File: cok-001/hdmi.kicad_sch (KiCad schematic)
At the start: 73 parts, among them J2501 HDMI_A, Q2502 DTA144E, Q2504 DTA144E, Q2507 DTC144E

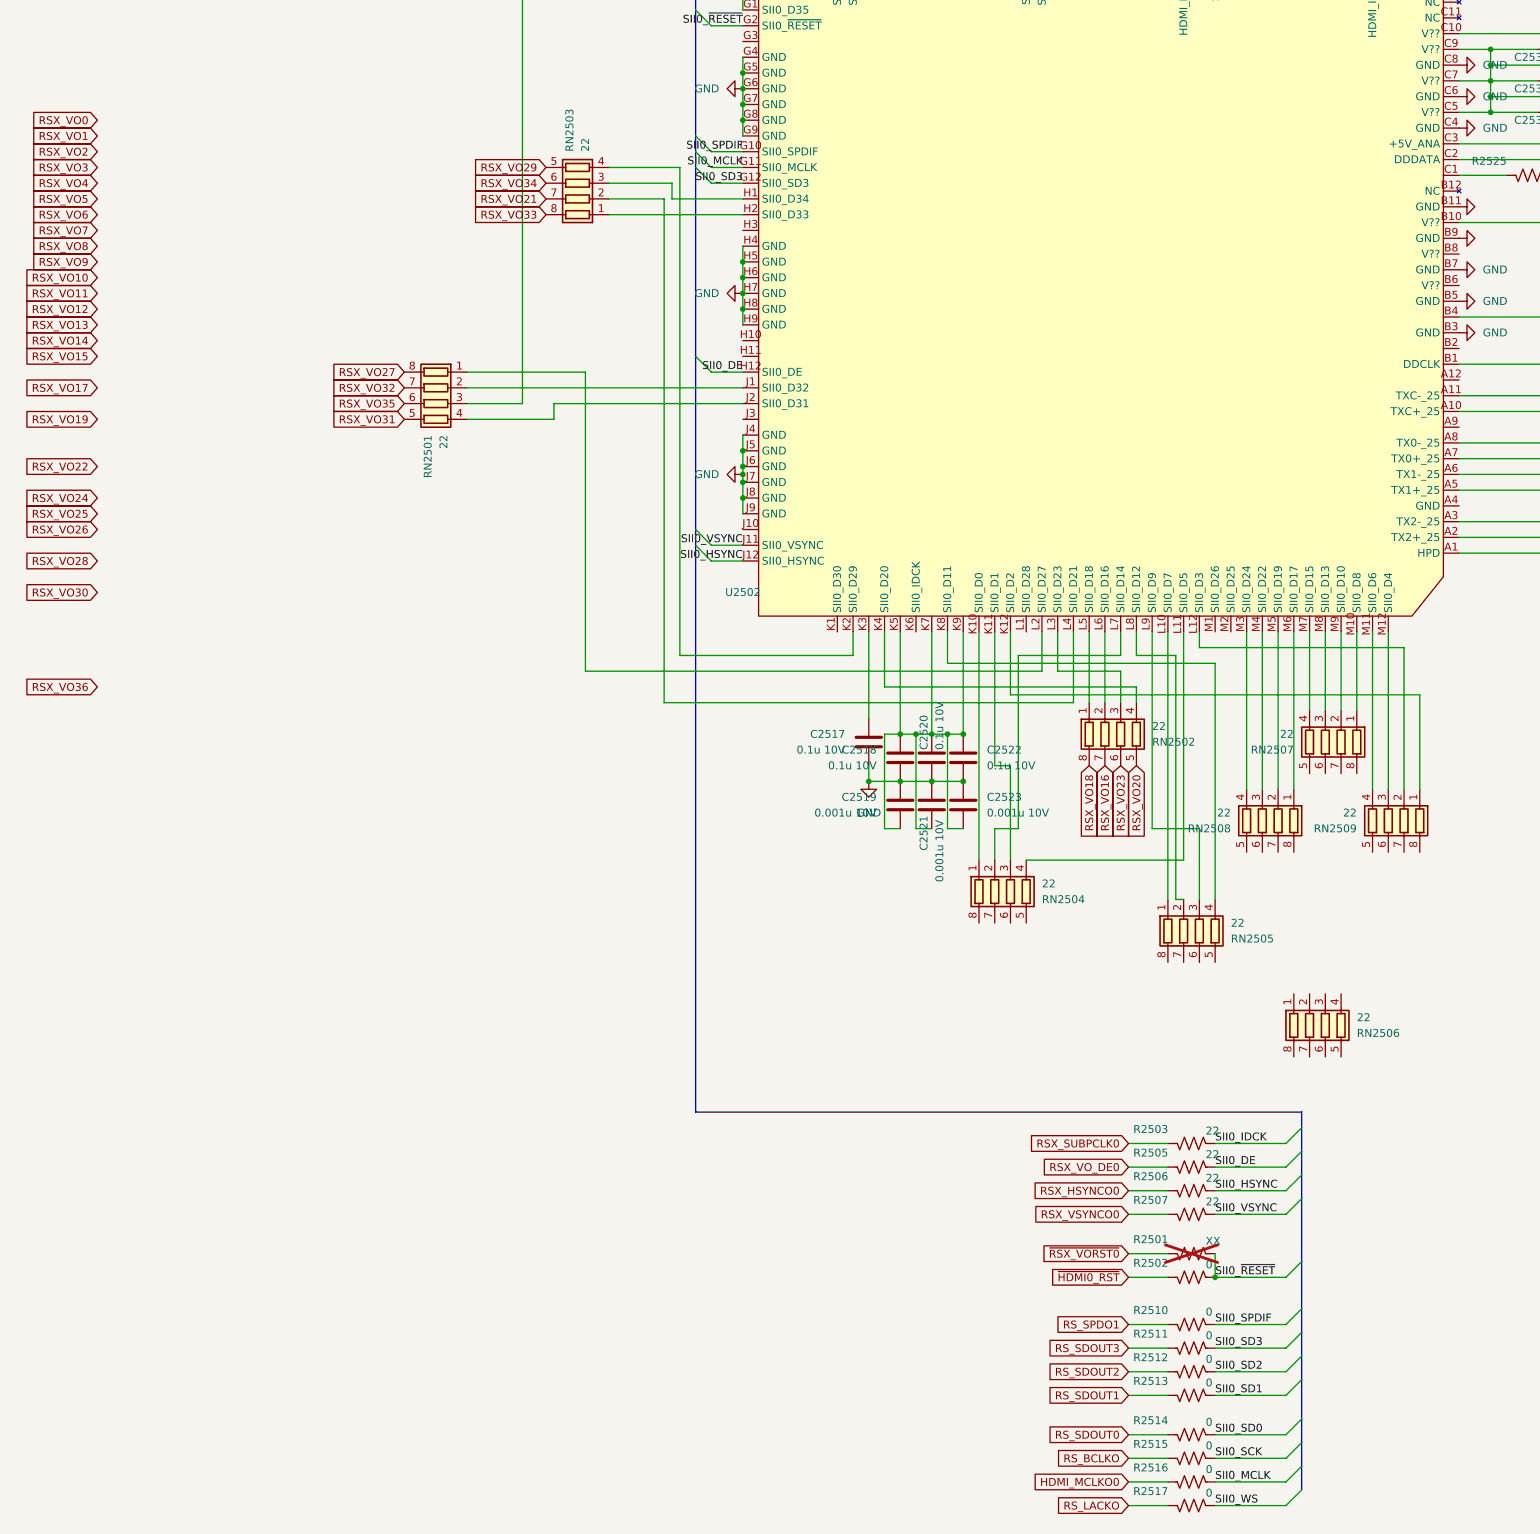
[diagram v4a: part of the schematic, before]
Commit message: hd sb
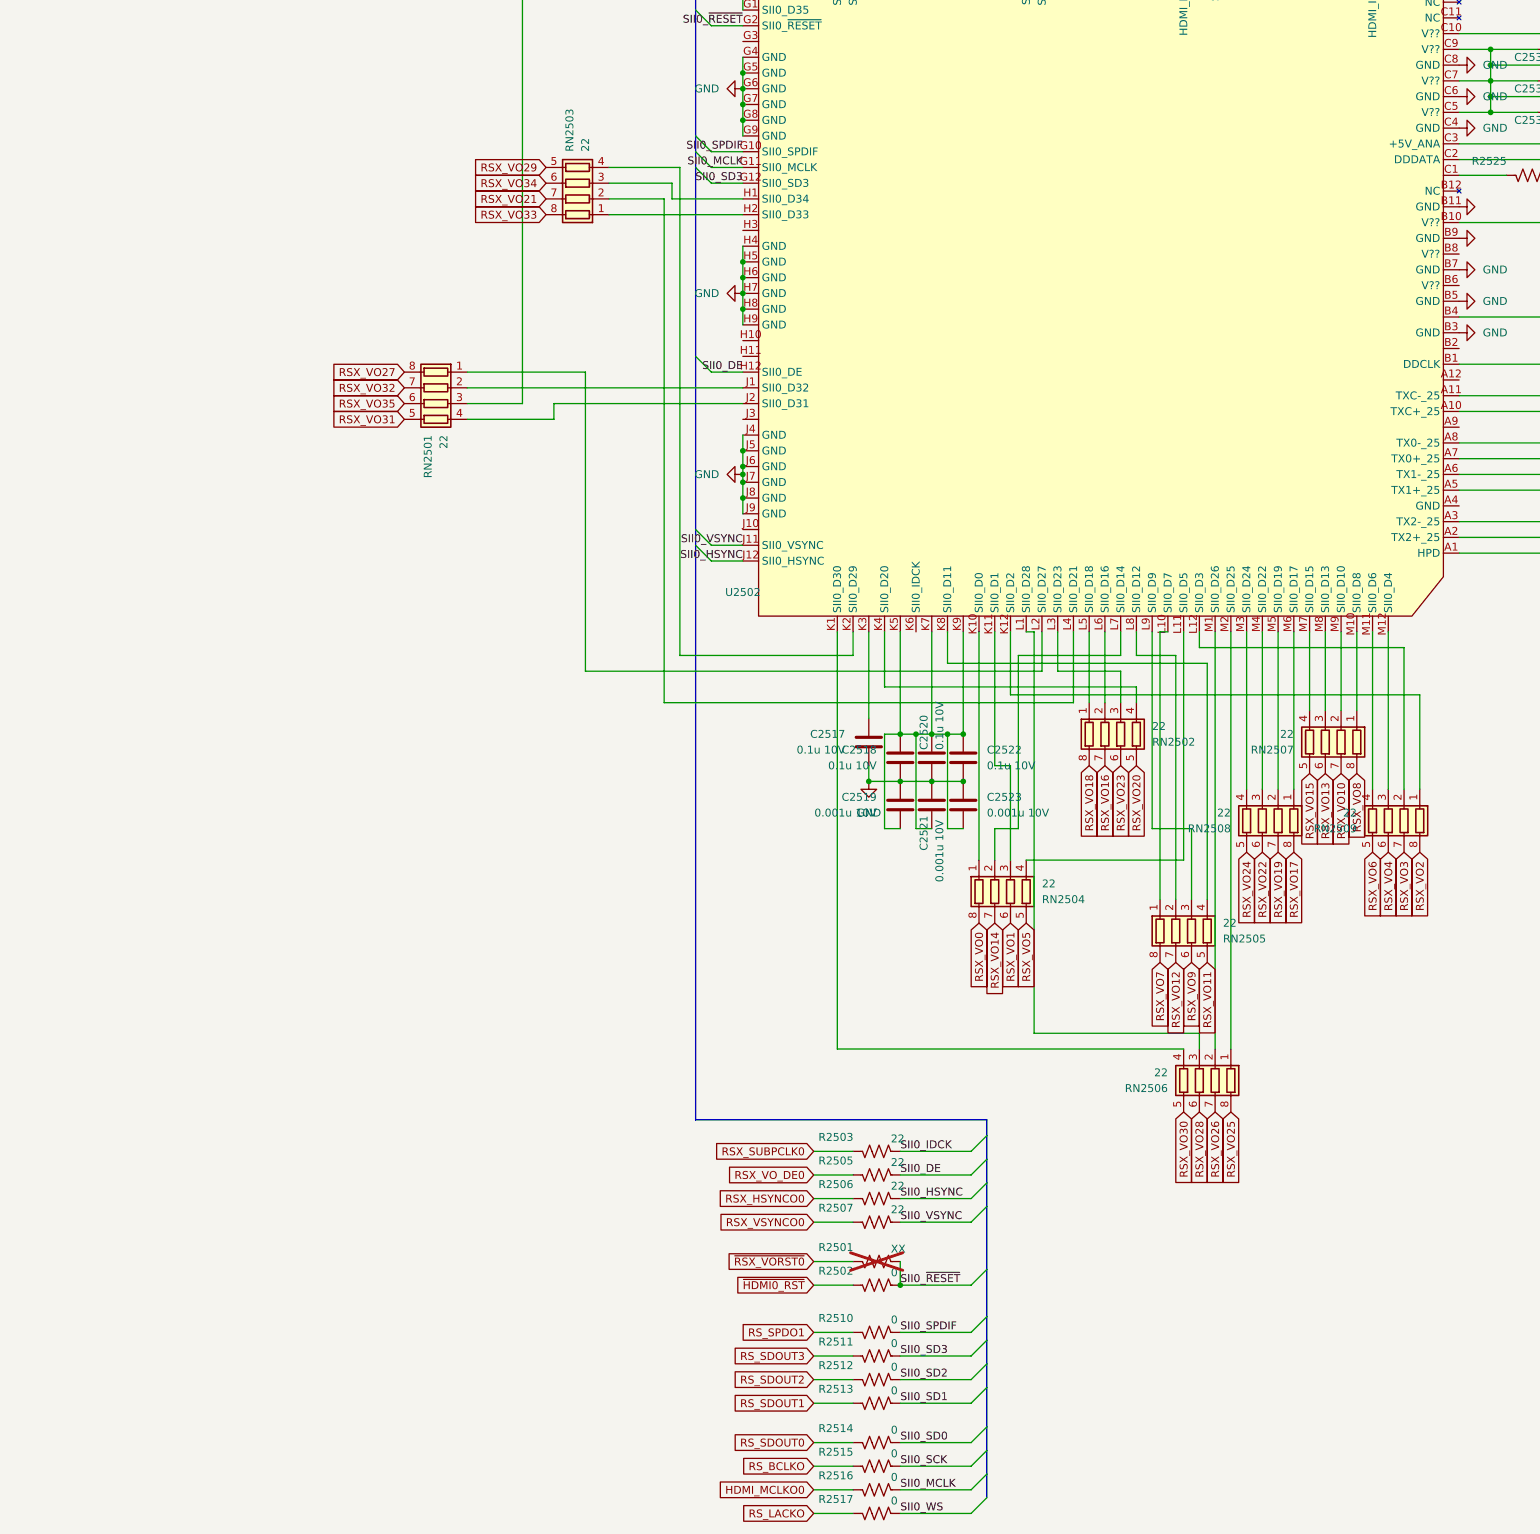
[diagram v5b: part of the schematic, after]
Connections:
- net RSX_VO0: now also RN2504.8 (R1.2)
- net RSX_VO1: now also RN2504.6 (R3.2)
- net RSX_VO10: now also RN2507.7 (R2.2)
- net RSX_VO11: now also RN2505.5 (R4.2)
- net RSX_VO12: now also RN2505.7 (R2.2)
- net RSX_VO13: now also RN2507.6 (R3.2)
- net RSX_VO14: now also RN2504.7 (R2.2)
- net RSX_VO15: now also RN2507.5 (R4.2)
- net RSX_VO17: now also RN2508.8 (R1.2)
- net RSX_VO19: now also RN2508.7 (R2.2)
- net RSX_VO2: now also RN2509.8 (R1.2)
- net RSX_VO22: now also RN2508.6 (R3.2)
- net RSX_VO24: now also RN2508.5 (R4.2)
- net RSX_VO25: now also RN2506.8 (R1.2)
- net RSX_VO26: now also RN2506.7 (R2.2)
- net RSX_VO28: now also RN2506.6 (R3.2)
- net RSX_VO3: now also RN2509.7 (R2.2)
- net RSX_VO30: now also RN2506.5 (R4.2)
- net RSX_VO4: now also RN2509.6 (R3.2)
- net RSX_VO5: now also RN2504.5 (R4.2)
- net RSX_VO6: now also RN2509.5 (R4.2)
- net RSX_VO7: now also RN2505.8 (R1.2)
- net RSX_VO8: now also RN2507.8 (R1.2)
- net RSX_VO9: now also RN2505.6 (R3.2)
- net at U2502.K1 (SII0_D30): now also RN2506.4 (R4.1)
- net at U2502.L1 (SII0_D28): now also RN2506.3 (R3.1)
- net at U2502.M1 (SII0_D26): now also RN2506.2 (R2.1)
- net at U2502.M2 (SII0_D25): now also RN2506.1 (R1.1)
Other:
- moved on the sheet: R2501, R2502, R2503, R2505, R2506, R2507, R2510, R2511, R2512, R2513, R2514, R2515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
